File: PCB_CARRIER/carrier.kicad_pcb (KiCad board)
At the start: 6 copper layers, 69.6 x 46 mm, 87 parts, among them J1 SODIMM-260_Split, J2 Micro_SD_Card_Det2, Q2 BSS138, Q3 BSS138, Q4 BC817-40, Q5 BSS138, SW1 SW_DIP_x04, U1 SN74LVC8T245, U2 SN74LVC8T245, U3 SN74LVC8T245, U4 RT9742GGJ5

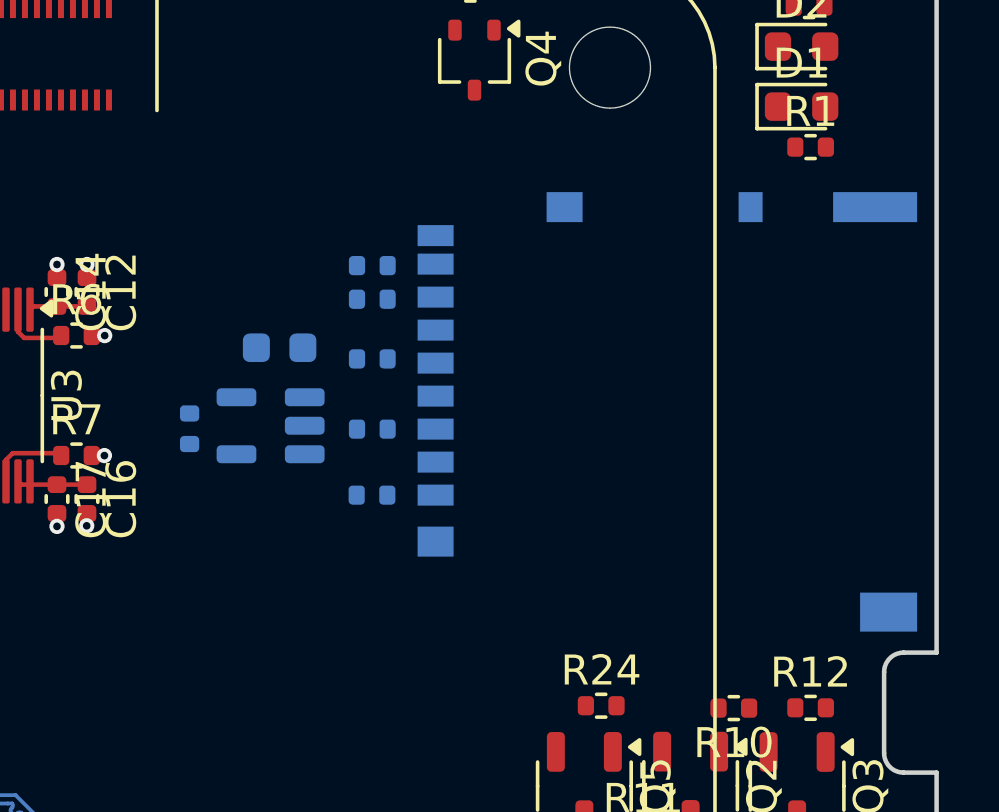
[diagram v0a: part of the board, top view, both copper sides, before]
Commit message: routing the SD card!
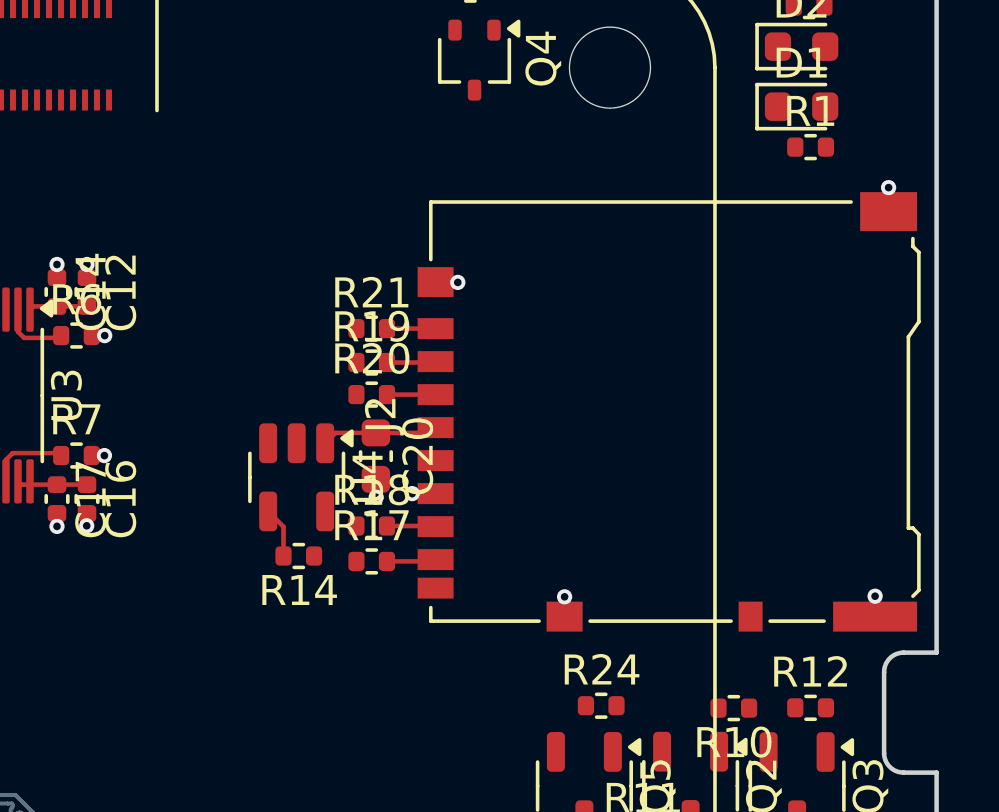
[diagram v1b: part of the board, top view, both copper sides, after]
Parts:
- C20, J2, R14, R17, R18, R19, R20, R21, U4: moved to F.Cu
- moved R17 9.86 mm to (150.8, 75.0), turned to 0 degrees
- moved R18 7.56 mm to (150.8, 73.8), turned to 0 degrees
- moved R14 5.59 mm to (148.3, 74.8), turned to 180 degrees
- moved R21 5.55 mm to (150.8, 67.2), turned to 0 degrees
- moved C20 4.83 mm to (150.9, 71.5), turned to -90 degrees
- moved U4 1.93 mm to (148.3, 72.2), turned to -90 degrees
- moved R20 1.15 mm to (150.8, 69.4), turned to 0 degrees
- moved R19 0.12 mm to (150.8, 68.3), turned to 0 degrees
- turned J2 to 90 degrees
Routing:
- net GND: track 122.3 -> 126.6 mm, vias 115 -> 121
- net SD_PWR: track 0.00 -> 3.90 mm
- net SD_PWR_ON: track 0.00 -> 1.70 mm
- net SD_DAT1: track 0.00 -> 1.64 mm
- net SD_DAT3: track 0.00 -> 1.63 mm
- net SD_DAT0: track 0.00 -> 1.63 mm
- net SD_DAT2: track 0.00 -> 1.62 mm
- net SD_CMD: track 0.00 -> 1.62 mm

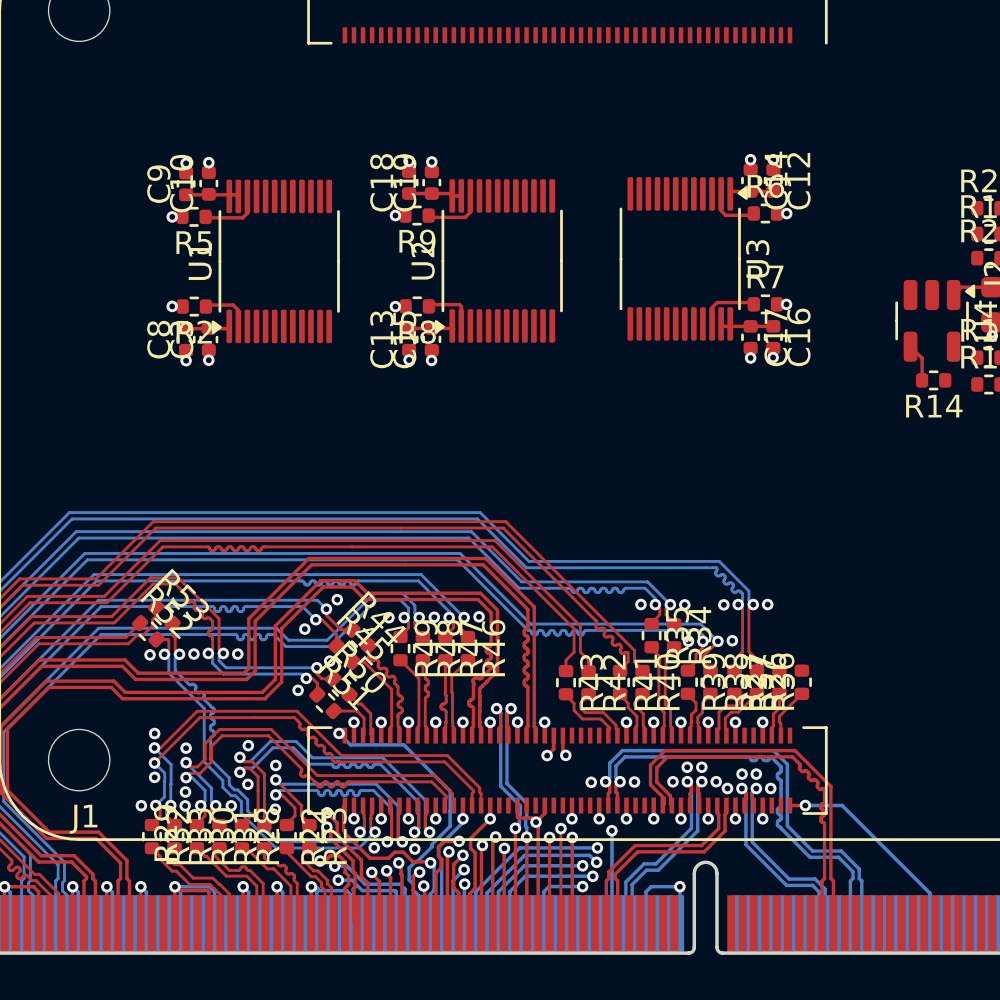
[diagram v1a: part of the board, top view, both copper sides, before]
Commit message: re-routing USB to have less crosstalk
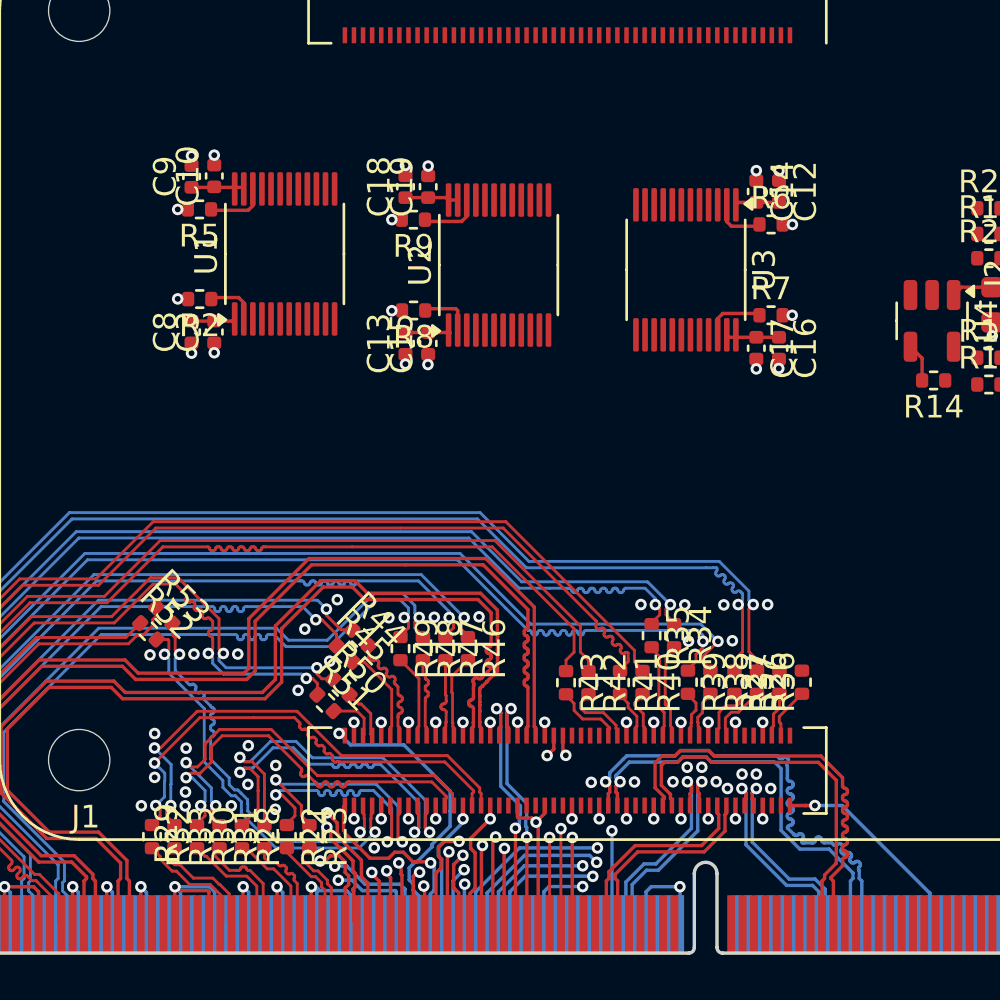
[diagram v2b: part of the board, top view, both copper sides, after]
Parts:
- moved C16 0.54 mm to (141.5, 73.4)
- moved C17 0.54 mm to (140.5, 73.4)
- moved C12 0.54 mm to (141.5, 66.5)
- moved C14 0.54 mm to (140.5, 66.5)
- moved R6 0.54 mm to (141.2, 67.9)
- moved R7 0.54 mm to (141.2, 71.9)
- moved U3 0.54 mm to (137.4, 69.9)
- moved U1 0.41 mm to (119.8, 69.2)
- moved C3 0.41 mm to (116.7, 72.6)
- moved C8 0.41 mm to (115.7, 72.6)
- moved R5 0.41 mm to (116.0, 67.2)
- moved C10 0.41 mm to (116.7, 65.8)
- moved C9 0.41 mm to (115.7, 65.8)
- moved R2 0.41 mm to (116.0, 71.2)
- moved C13 0.24 mm to (125.1, 73.2)
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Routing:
- net USB3-0-TX_P: track 19.5 -> 22.1 mm
- net USB3-0-RX_P: track 17.0 -> 19.1 mm
- net USB3-0-TX_N: track 19.4 -> 18.3 mm
